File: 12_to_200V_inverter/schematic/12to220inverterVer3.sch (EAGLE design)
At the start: 255 parts, among them IC1 UC3842, IC10 TL494, IC2 PC817, IC3 LM358, IC4 TL431, IC5 LM317, IC6 74HC595, IC7 74HC595, IC8 ATTINY45, IC9 TL431, J100 0, J101 0, J2 0, J3 0, T10 16N60, T11 BC847, T12 BC847, T13 AO3401, T14 AO3401, T15 BC847, T16 BSS84, T17 BC847, T18 BC847, T19 BSS84, T2 IRF830, T21 BC847, T22 BC847, T23 BSS84, T24 BC847, T3 IRF830, T4 BC847, T5 BC857, T6 BC857, T7 IRFZ24N, T8 IRFZ24N, T9 BC857, U100 DF06S, X1 BAT+, X2 LAMP1, X3 LAMP1, X4 BAT-, X5 220VAC, X6 LAMP1_SWITCH, X7 LAMP1_SWITCH, X8 MCU_PROGRAMMING

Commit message: 12 to 200V inverter. New board with ETD transformers. Finally routed.
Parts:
- IC4: device __MyCommonLib1:TL431TO-92A_PINS_SWAPPED -> __MyCommonLib1:TL431TO-92A
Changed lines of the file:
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@@
 <setting verticaltext="up"/>
 </settings>
-<grid distance="0.05" unitdist="inch" unit="inch" style="lines" multiple="2" display="yes" altdistance="0.01" altunitdist="inch" altunit="inch"/>
+<grid distance="0.1" unitdist="inch" unit="inch" style="lines" multiple="1" display="no" altdistance="0.01" altunitdist="inch" altunit="inch"/>
 <layers>
 <layer number="1" name="Top" color="4" fill="1" visible="yes" active="no"/>
@@
 <part name="L1" library="__MyCommonLib1" deviceset="L" device="(7MM)" value="20uH"/>
 <part name="CE3" library="__MyCommonLib1" deviceset="CE" device="6.3MM" value="47uF x 25V"/>
-<part name="IC4" library="__MyCommonLib1" deviceset="TL431" device="TO-92A_PINS_SWAPPED" value="TL431"/>
+<part name="IC4" library="__MyCommonLib1" deviceset="TL431" device="TO-92A" value="TL431"/>
 <part name="R59" library="__MyCommonLib1" deviceset="R" device="SMD_0805" value="5K6"/>
 <part name="R61" library="__MyCommonLib1" deviceset="R" device="SMD_0805" value="10K"/>

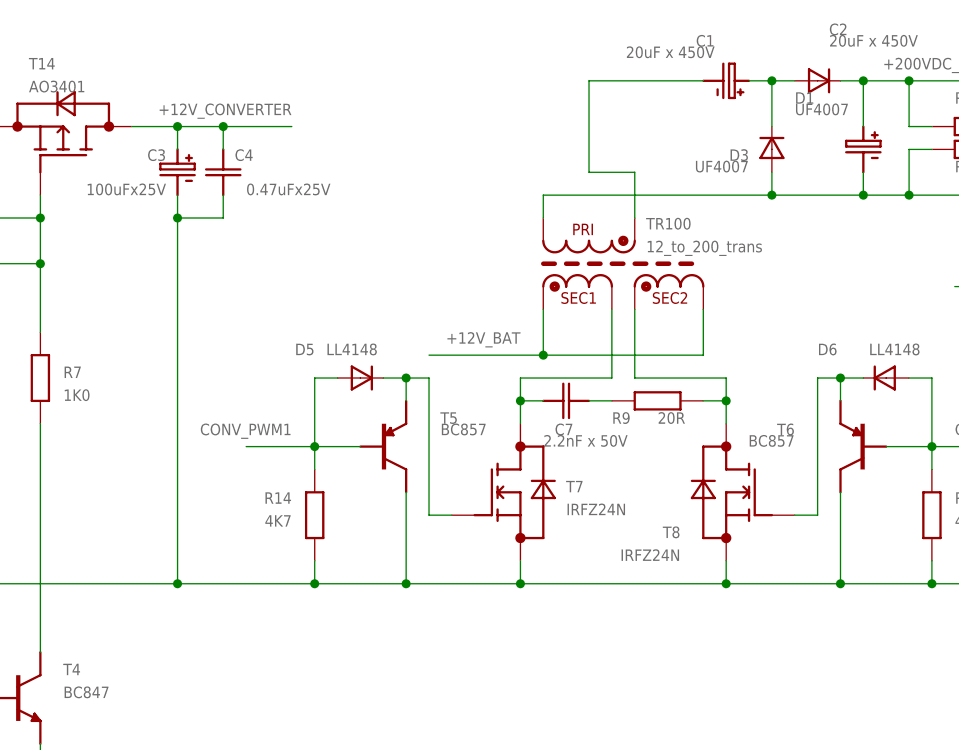
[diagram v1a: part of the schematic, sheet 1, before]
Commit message: 12 to 200V inverter. New board with ETD transformers. Finally routed.
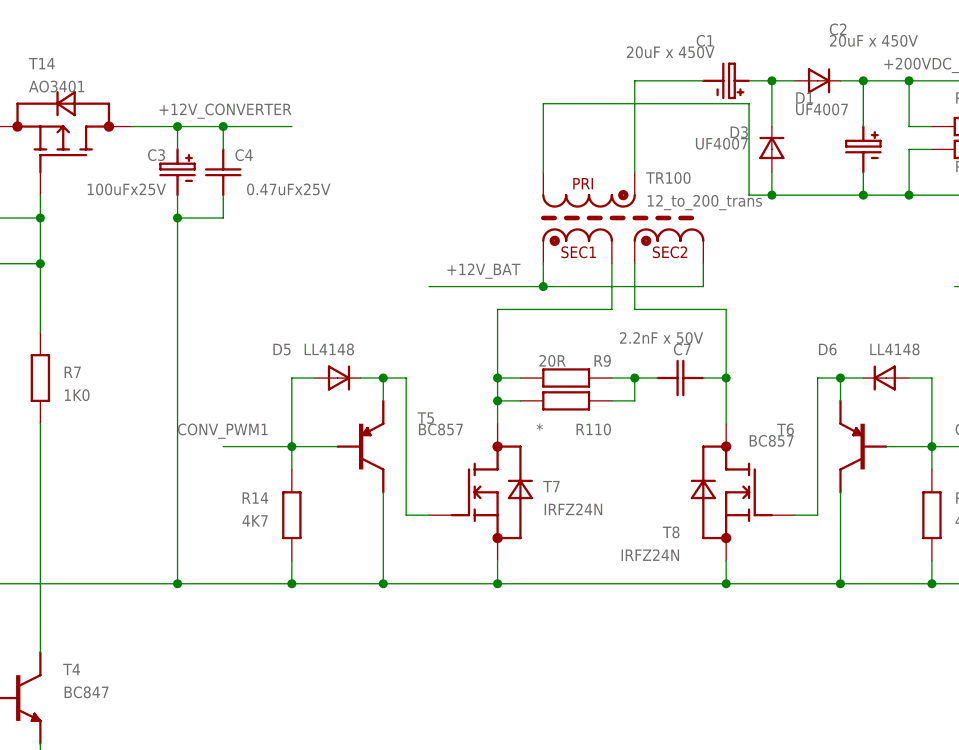
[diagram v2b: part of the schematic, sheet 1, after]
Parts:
- added R110: *, __MyCommonLib1:RSMD_1206
- F2: device __MyCommonLib1:FUSE20X5.6MM -> __MyCommonLib1:FUSE(20X5MM_VERT_WIRE)
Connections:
- net N$24: now also R110.PIN0, R9.PIN0; no longer C7.PIN1
- net N$25: now also C7.PIN1; no longer R9.PIN0
- net N$26: now also R110.PIN1
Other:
- moved on the sheet: C7, D5, R14, R9, T5, T7, TR100
